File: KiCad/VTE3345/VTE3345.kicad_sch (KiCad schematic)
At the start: 26 parts, among them J1 Program, J2 Keypad, J3 Display, J4 Power, Q1 IRF540N, Q2 BD138, SW1 Reset, SW2 Mode, SW3 Switch, U1 ESP-12F, U2 AMS1117-3.3

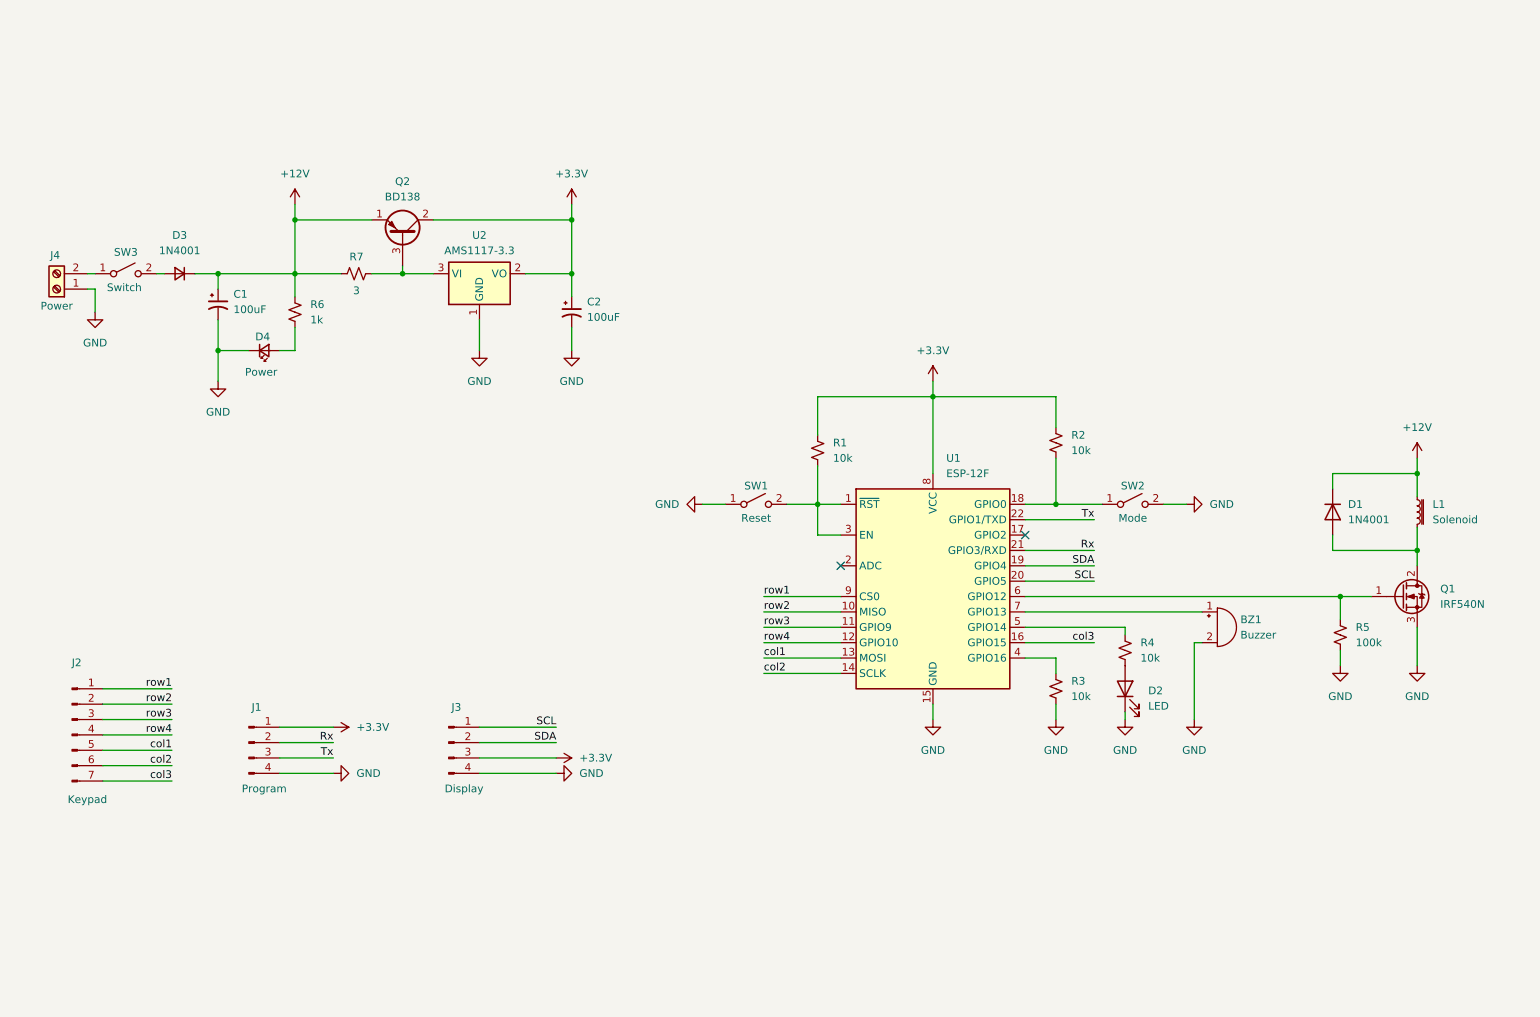
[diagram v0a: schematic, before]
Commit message: Updates
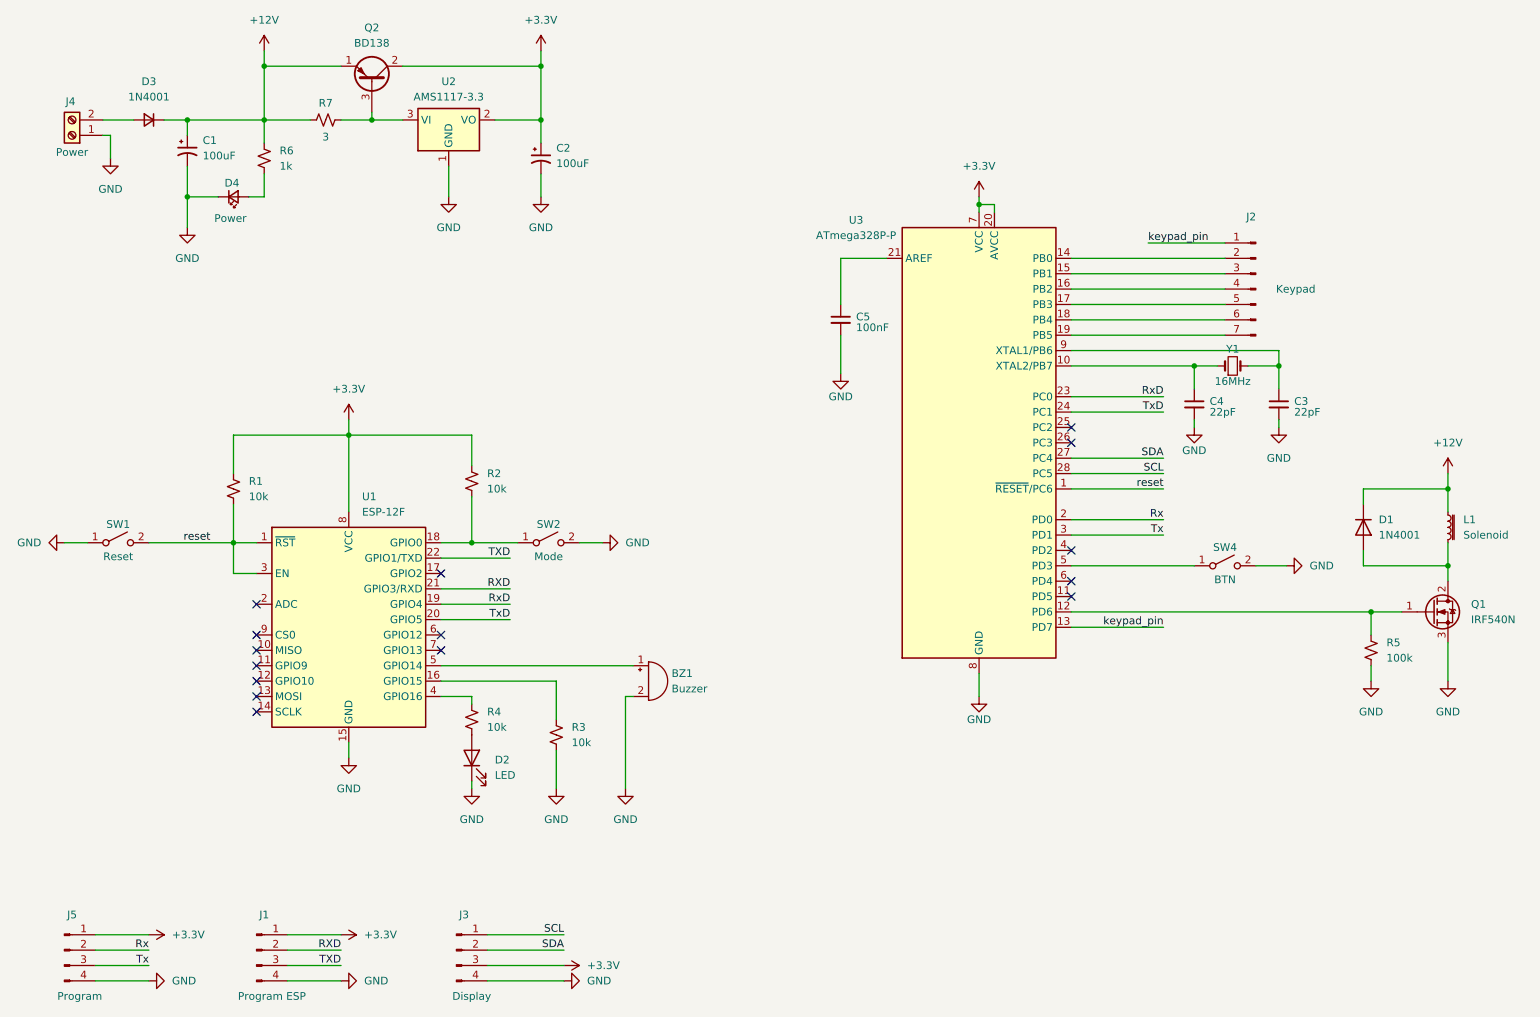
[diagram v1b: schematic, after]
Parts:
- removed SW3: Switch, TestPoint:TestPoint_2Pads_Pitch2.54mm_Drill0.8mm, symbol Switch:SW_SPST
- added C3, C4: 22pF, Capacitor_THT:C_Disc_D3.0mm_W1.6mm_P2.50mm, symbol Device:C_Small
- added C5: 100nF, Capacitor_THT:C_Disc_D3.0mm_W1.6mm_P2.50mm, symbol Device:C_Small
- added J5: Program, Connector_PinHeader_2.54mm:PinHeader_1x04_P2.54mm_Vertical, symbol Connector:Conn_01x04_Pin
- added SW4: BTN, TestPoint:TestPoint_2Pads_Pitch2.54mm_Drill0.8mm, symbol Switch:SW_SPST
- added U3: ATmega328P-P, Package_DIP:DIP-28_W7.62mm_LongPads, symbol MCU_Microchip_ATmega:ATmega328P-P
- added Y1: 16MHz, Crystal:Crystal_HC52-U_Vertical, symbol Device:Crystal_Small
- J1: value Program -> Program ESP
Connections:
- net +3.3V: now also J5.1 (Pin_1), U3.20 (AVCC), U3.7 (VCC)
- net GND: now also C3.2, C4.2, C5.2, J5.4 (Pin_4), SW4.2 (B), U3.22 (GND), U3.8 (GND)
- net Rx: now also J5.2 (Pin_2), U3.2 (PD0); no longer J1.2 (Pin_2), U1.21 (GPIO3/RXD)
- net SCL: now also U3.28 (PC5); no longer U1.20 (GPIO5)
- net SDA: now also U3.27 (PC4); no longer U1.19 (GPIO4)
- net Tx: now also J5.3 (Pin_3), U3.3 (PD1); no longer J1.3 (Pin_3), U1.22 (GPIO1/TXD)
- net at D3.2 (A): now also J4.2 (Pin_2)
- net reset: now reaches R1.2, SW1.2 (B), U1.1 (~{RST}), U1.3 (EN)
- net reset: now also U3.1 (~{RESET}/PC6)
- net at BZ1.1 (+): now also U1.5 (GPIO14); no longer U1.7 (GPIO13)
- net at Q1.1 (G), R5.2: now also U3.12 (PD6); no longer U1.6 (GPIO12)
- net at R3.1: now also U1.16 (GPIO15); no longer U1.4 (GPIO16)
- net at R4.1: now also U1.4 (GPIO16); no longer U1.5 (GPIO14)
- net col1: no longer names the net of U1.13 (MOSI)
- net col1: no longer J2.5 (Pin_5)
- net col2: no longer names the net of U1.14 (SCLK)
- net col2: no longer J2.6 (Pin_6)
- net col3: no longer names the net of J2.7 (Pin_7)
- net col3: now also U3.19 (PB5); no longer U1.16 (GPIO15)
- net row1: no longer names the net of U1.9 (CS0)
- net row1: no longer J2.1 (Pin_1)
- net row2: no longer names the net of U1.10 (MISO)
- net row2: no longer J2.2 (Pin_2)
- net row3: no longer names the net of U1.11 (GPIO9)
- net row3: no longer J2.3 (Pin_3)
- net row4: no longer names the net of U1.12 (GPIO10)
- net row4: no longer J2.4 (Pin_4)
- new net: C5.1, U3.21 (AREF)
- new net: SW4.1 (A), U3.5 (PD3)
- new net: C4.1, U3.10 (XTAL2/PB7), Y1.1
- new net: C3.1, U3.9 (XTAL1/PB6), Y1.2
- new net: J2.2 (Pin_2), U3.14 (PB0)
- new net: J2.3 (Pin_3), U3.15 (PB1)
- new net: J2.4 (Pin_4), U3.16 (PB2)
- new net: J2.5 (Pin_5), U3.17 (PB3)
- new net: J2.6 (Pin_6), U3.18 (PB4)
- new net RXD: J1.2 (Pin_2), U1.21 (GPIO3/RXD)
- new net RxD: U1.19 (GPIO4), U3.23 (PC0)
- new net TXD: J1.3 (Pin_3), U1.22 (GPIO1/TXD)
- new net TxD: U1.20 (GPIO5), U3.24 (PC1)
- new net keypad_pin: J2.1 (Pin_1), U3.13 (PD7)
- no-connect marks 2 -> 15
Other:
- moved on the sheet: BZ1, C1, C2, D1, D2, D3, D4, J1, J2, J3, J4, L1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
